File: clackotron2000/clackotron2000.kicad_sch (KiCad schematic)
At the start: 58 parts, among them J3 Conn_ESP_Prog, J4 Power, J5 Output, J6 Conn_01x04, Q1 BSN20, Q2 BSN20, Q3 BSN20, Q4 BSN20, SW1 SW_Push_DPDT, SW2 SW_Push, SW3 SW_Push, U1 ESP32-WROOM-32, U2 SP3485EN, U3 R-78B5.0-1.0, U4 PCF85263ATT, U5 AMS1117-3.3, Y1 Crystal

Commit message: chore: rebase changes from internal repository
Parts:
- U3: digikey (none) -> R-78K5.0-0.5
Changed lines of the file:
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@@
+      (effects (font (size 1.27 1.27)) hide)
+    )
+    (property "digikey" "R-78K5.0-0.5" (at 182.88 31.75 0)
       (effects (font (size 1.27 1.27)) hide)
     )

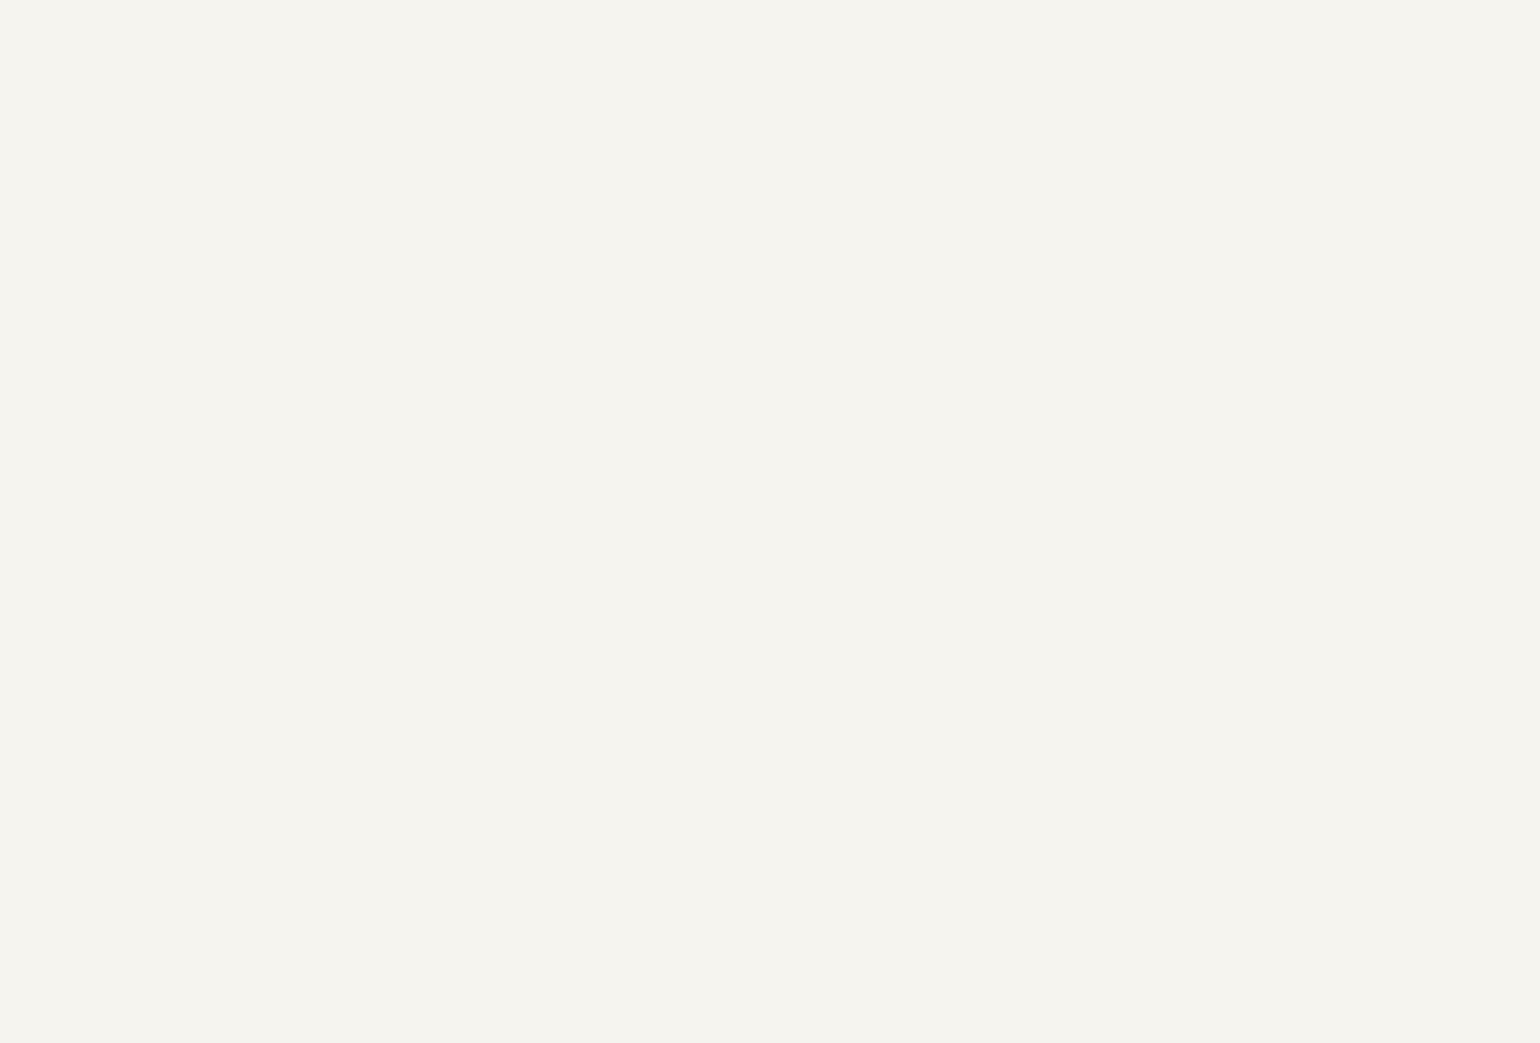
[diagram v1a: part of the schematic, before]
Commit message: add new parts for next hardware revision to schematic
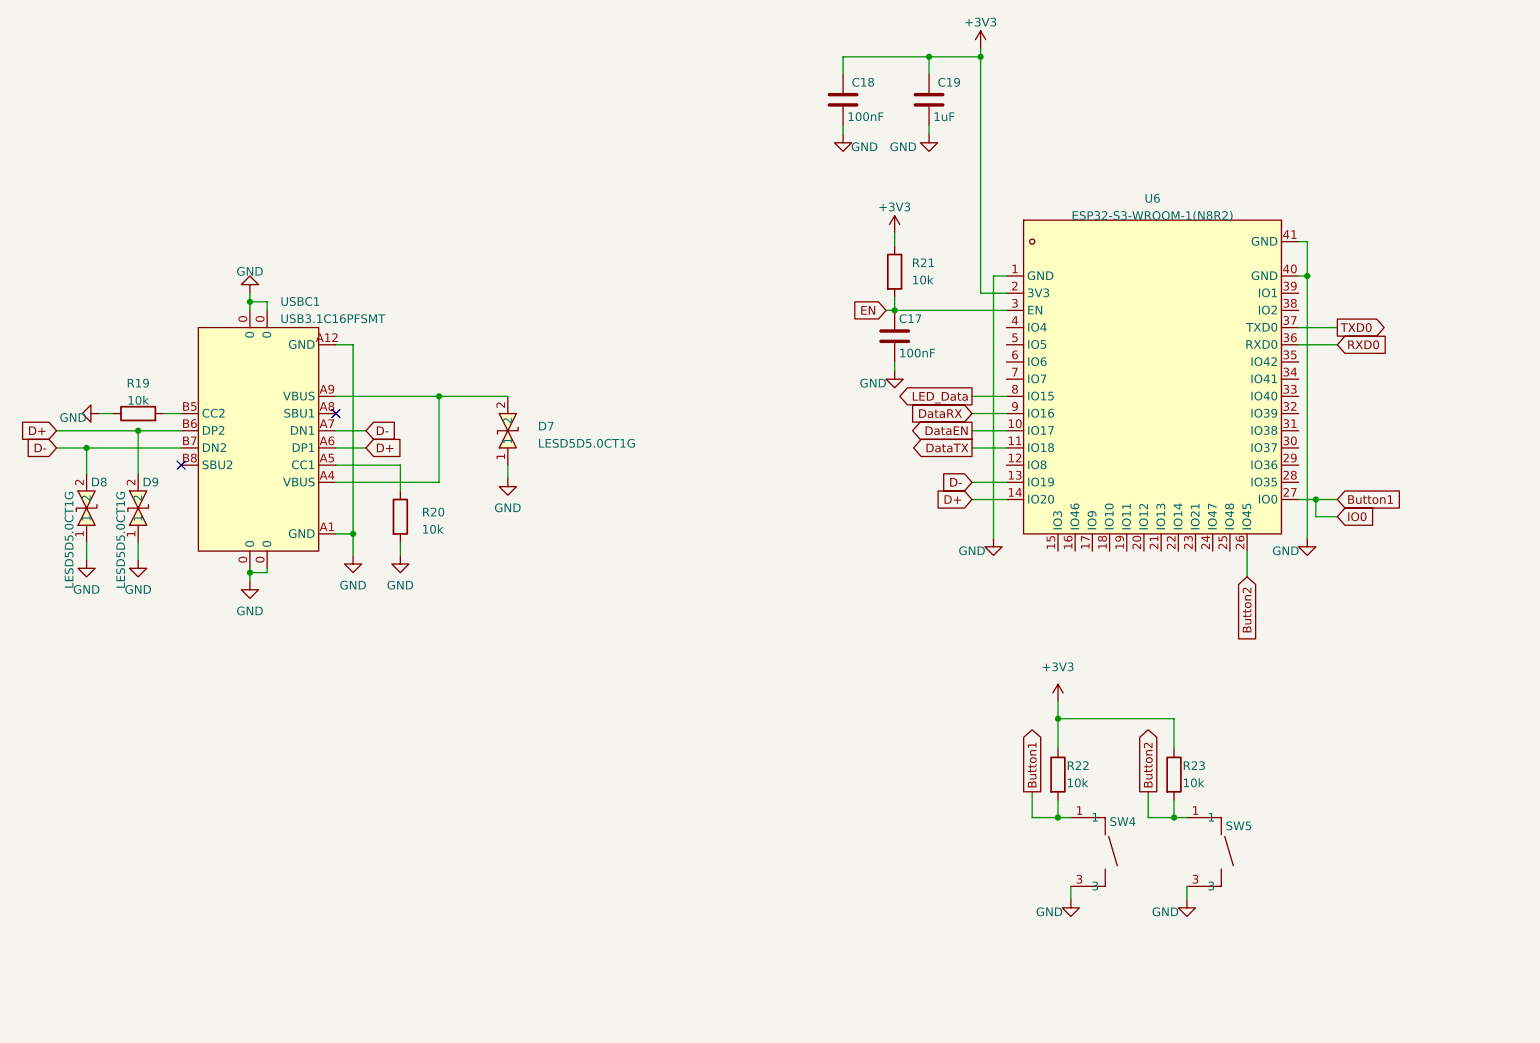
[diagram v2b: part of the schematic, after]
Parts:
- added C17, C18: 100nF, Capacitor_SMD:C_0805_2012Metric, symbol Device:C
- added C19: 1uF, Capacitor_SMD:C_0805_2012Metric, symbol Device:C
- added D7, D8, D9: LESD5D5.0CT1G, clackotron_fp:SOD-523_L1.2-W0.8-LS1.6-BI, symbol clackotronlib:LESD5D5.0CT1G
- added R19, R20, R21, R22, R23: 10k, Resistor_SMD:R_0805_2012Metric, symbol Device:R
- added SW4, SW5: K2-1102SP-C4SC-04, clackotron_fp:KEY-SMD_4P-L6.0-W6.0-P4.50-LS9.5-BL, symbol clackotronlib:K2-1102SP-C4SC-04
- added U6: ESP32-S3-WROOM-1(N8R2), clackotron_fp:WIRELM-SMD_ESP32-S3-WROOM-1, symbol clackotronlib:ESP32-S3-WROOM-1(N8R2)
- added USBC1: USB3.1C16PFSMT, clackotron_fp:USB-C-SMD_TYPE-C-USB-17, symbol clackotronlib:USB3.1C16PFSMT
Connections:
- net IO0 is gone; now on net Button1: J3.3 (Pin_3), U1.25 (IO0)
- net +3V3: now also C18.1, C19.1, R21.1, R22.1, R23.1, U6.2 (3V3)
- net Button1: now also R22.2, SW4.1, SW4.2, U6.27 (IO0)
- net Button2: now also R23.2, SW5.1, SW5.2, U6.26 (IO45)
- net DataEN: now also U6.10 (IO17)
- net DataRX: now also U6.9 (IO16)
- net DataTX: now also U6.11 (IO18)
- net EN: now also C17.1, R21.2, U6.3 (EN)
- net GND: now also C17.2, C18.2, C19.2, D7.1, D8.1, D9.1, R19.1, R20.2, SW4.3, SW4.4, SW5.3, SW5.4, U6.1 (GND), U6.40 (GND), U6.41 (GND), USBC1.0, USBC1.A1 (GND), USBC1.A12 (GND)
- net LED_Data: now also U6.8 (IO15)
- net RXD0: now also U6.36 (RXD0)
- net TXD0: now also U6.37 (TXD0)
- new net: D7.2, USBC1.A4 (VBUS), USBC1.A9 (VBUS)
- new net: R20.1, USBC1.A5 (CC1)
- new net: R19.2, USBC1.B5 (CC2)
- new net D+: D9.2, U6.14 (IO20), USBC1.A6 (DP1), USBC1.B6 (DP2)
- new net D-: D8.2, U6.13 (IO19), USBC1.A7 (DN1), USBC1.B7 (DN2)
- no-connect marks 19 -> 21
